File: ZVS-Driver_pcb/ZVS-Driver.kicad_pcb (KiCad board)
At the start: 2 copper layers, 163 x 96.2 mm, 25 parts, among them J1 Screw_Terminal_01x02, J3 Screw_Terminal_01x04, Q1 IRF540N, Q2 IRF540N, Q3 IRF540N, Q4 IRF540N, Q5 IRF540N

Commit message: Mosfet fix
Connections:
- Q2 pad 2: 0 -> Net-(D6-K)
- Q2 pad 3: Net-(D6-K) -> 0
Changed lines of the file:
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@@
 			(layers "*.Cu" "*.Mask")
 			(remove_unused_layers no)
-			(net 3 "0")
+			(net 1 "Net-(D6-K)")
 			(pinfunction "D")
 			(pintype "passive")
@@
 			(layers "*.Cu" "*.Mask")
 			(remove_unused_layers no)
-			(net 1 "Net-(D6-K)")
+			(net 3 "0")
 			(pinfunction "S")
 			(pintype "passive")

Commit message: new millennium falcon design and colors for the pcb
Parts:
- added G***: LOGO, LOGO, F.Cu at (100.0, 93.0)
- moved R6 34.0 mm to (49.0, 71.6), turned to 180 degrees
- moved J1 27.7 mm to (79.3, 38.9)
- moved Q3 25.3 mm to (47.7, 113.8)
- moved R1 13.4 mm to (86.7, 116.2)
- moved J3 8.39 mm to (64.3, 119.7)
- moved Q2 0.53 mm to (125.2, 116.4)
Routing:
- net Net-(D4-K): track 303.9 -> 240.7 mm
- net Net-(D4-A): track 85.9 -> 66.6 mm
- net Net-(D1-A): track 186.1 -> 194.9 mm
- net Net-(D3-K): track 250.8 -> 245.2 mm
- net Net-(Q3-D): track 48.8 -> 43.9 mm
- net 0: track 307.0 -> 303.7 mm
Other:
- board size 163 x 96.2 mm -> 258.8 x 119 mm

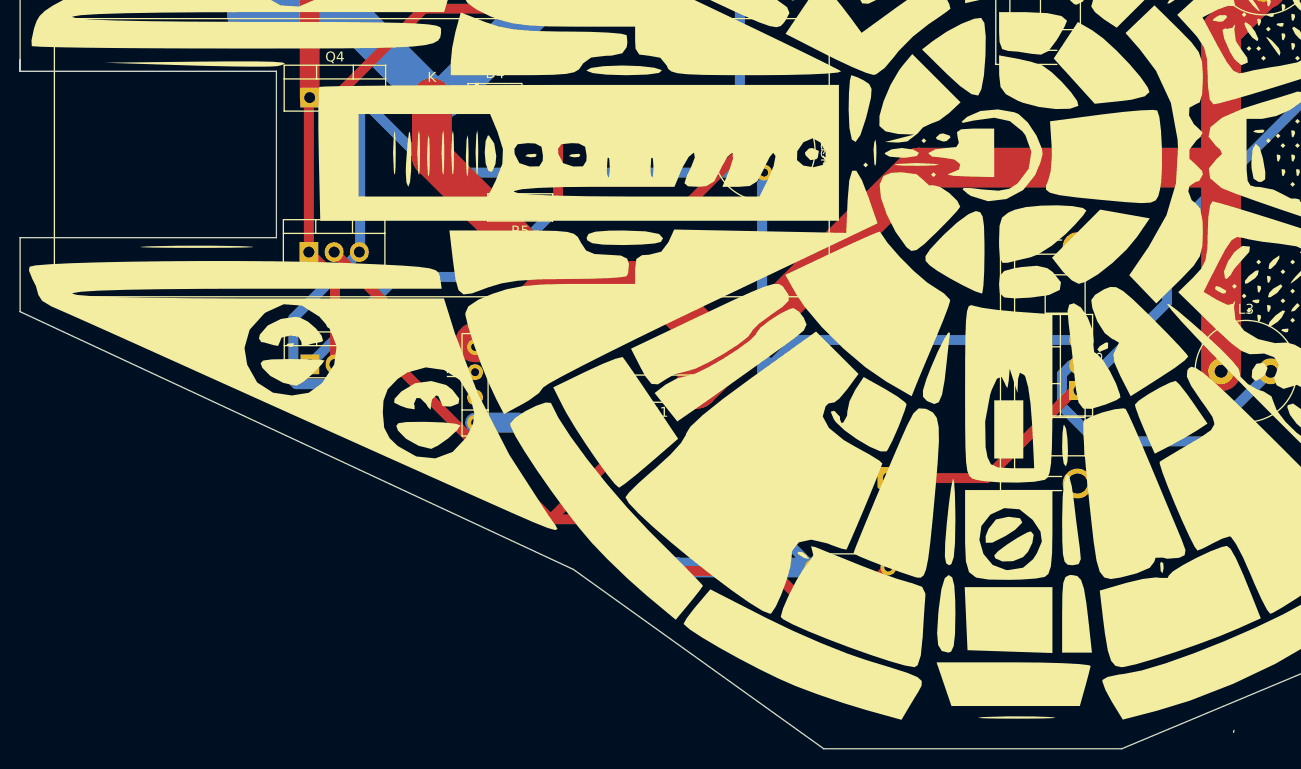
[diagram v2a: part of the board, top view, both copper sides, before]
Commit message: Fixes
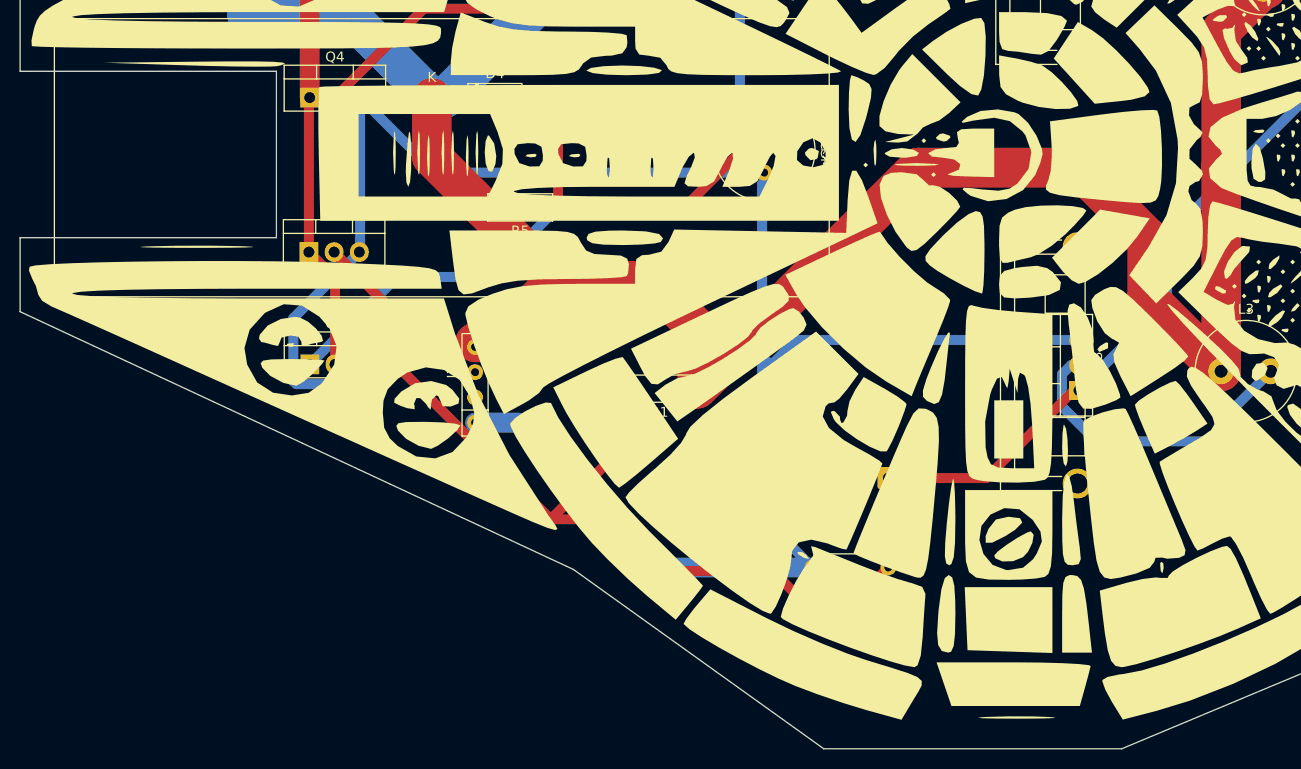
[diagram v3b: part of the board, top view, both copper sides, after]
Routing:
- net Net-(D4-K): track 240.7 -> 252.8 mm
- net 0: track 303.7 -> 302.2 mm
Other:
- outline, holes or cut-outs redrawn
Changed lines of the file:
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@@
-	)
-	(gr_line
-		(start 18.55 83.15)
-		(end 18.55 84.3)
-		(stroke
-			(width 0.05)
-			(type default)
-		)
-		(layer "Edge.Cuts")
-	)
-	(gr_line
-		(start 140.7 150.85)
-		(end 140.75 150.65)
-		(stroke
-			(width 0.05)
-			(type default)
-		)
-		(layer "Edge.Cuts")
 	)
 	(gr_line
@@
 			(keep_text_aligned yes)
 		)
-		(gr_text "12.5"
+		(gr_text "12,5"
 			(at 167.05 77.25 90)
 			(layer "User.1")
@@
 			(keep_text_aligned yes)
 		)
-		(gr_text "4.75"
+		(gr_text "4,75"
 			(at 110.05 62.125 90)
 			(layer "User.1")
@@
 			(keep_text_aligned yes)
 		)
-		(gr_text "4.75"
+		(gr_text "4,75"
 			(at 110.05 122.875 90)
 			(layer "User.1")
@@
 			(keep_text_aligned yes)
 		)
-		(gr_text "12.5"
+		(gr_text "12,5"
 			(at 168.55 108.25 90)
 			(layer "User.1")
@@
 	)
 	(segment
-		(start 98.33 134.25)
-		(end 83.25 134.25)
-		(width 2)
-		(layer "B.Cu")
-		(net 3)
-	)
-	(segment
 		(start 93.25 95.65)
 		(end 93.25 113)
@@
 	(segment
 		(start 83.25 134.25)
+		(end 98.33 134.25)
+		(width 2)
+		(layer "B.Cu")
+		(net 3)
+	)
+	(segment
+		(start 83.25 134.25)
 		(end 68.67 119.67)
 		(width 2)
@@
 	)
 	(segment
-		(start 84.75 134.25)
-		(end 83.25 134.25)
-		(width 2)
-		(layer "B.Cu")
-		(net 3)
-	)
-	(segment
 		(start 72.7 98)
 		(end 72.7 87)
@@
 	)
 	(segment
+		(start 125 94)
+		(end 108.96 94)
+		(width 4)
+		(layer "F.Cu")
+		(net 7)
+	)
+	(segment
 		(start 81.95 105.4)
 		(end 86.71 110.16)
@@
 	)
 	(segment
+		(start 132 107.05)
+		(end 132 101)
+		(width 4)
+		(layer "F.Cu")
+		(net 7)
+	)
+	(segment
 		(start 79.3 53.0625)
 		(end 78.8275 53.0625)
@@
 	)
 	(segment
+		(start 139.45 114.5)
+		(end 132 107.05)
+		(width 4)
+		(layer "F.Cu")
+		(net 7)
+	)
+	(segment
 		(start 60 92.92)
 		(end 65.08 98)
@@
 	)
 	(segment
-		(start 139.45 94)
-		(end 108.96 94)
-		(width 4)
-		(layer "F.Cu")
-		(net 7)
-	)
-	(segment
 		(start 143.7 76)
 		(end 139.45 80.25)
@@
 		(width 4)
 		(layer "F.Cu")
+		(net 7)
+	)
+	(segment
+		(start 132 101)
+		(end 125 94)
+		(width 4)
+		(layer "F.Cu")

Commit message: Silkscreen
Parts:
- added G***: LOGO, Library:doodles, F.Cu at (107.8, 91.9)
- G***: moved to B.Cu
- moved J1 103.2 mm to (75.0, 142.0)
- moved J3 64.3 mm to (121.0, 150.0), turned to 180 degrees
- turned G*** to -90 degrees
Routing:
- net Net-(D4-K): track 252.8 -> 308.1 mm
- net 0: track 302.2 -> 331.9 mm
- net Net-(D3-K): track 245.2 -> 245.8 mm
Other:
- board size 258.8 x 119 mm -> 258.8 x 119.1 mm
